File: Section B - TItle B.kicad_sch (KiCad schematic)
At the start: 2 parts

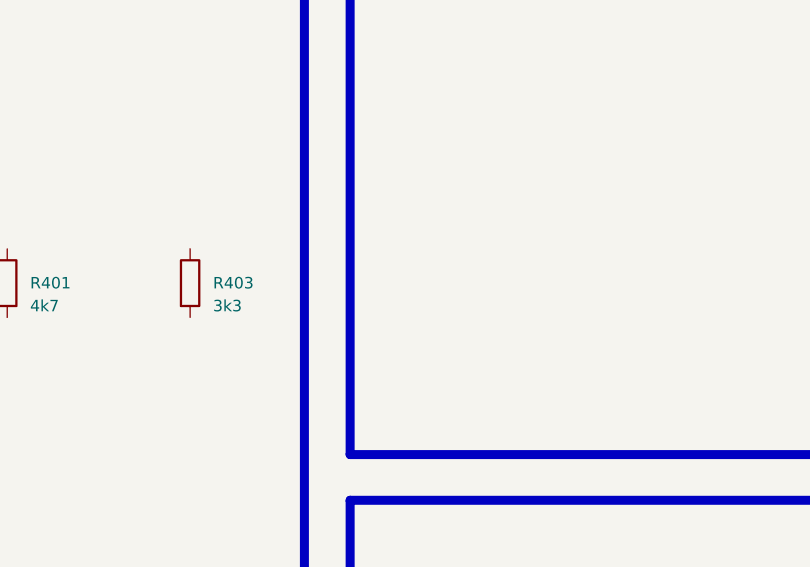
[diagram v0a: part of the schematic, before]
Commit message: section-a: grant myself all sheets, edit B
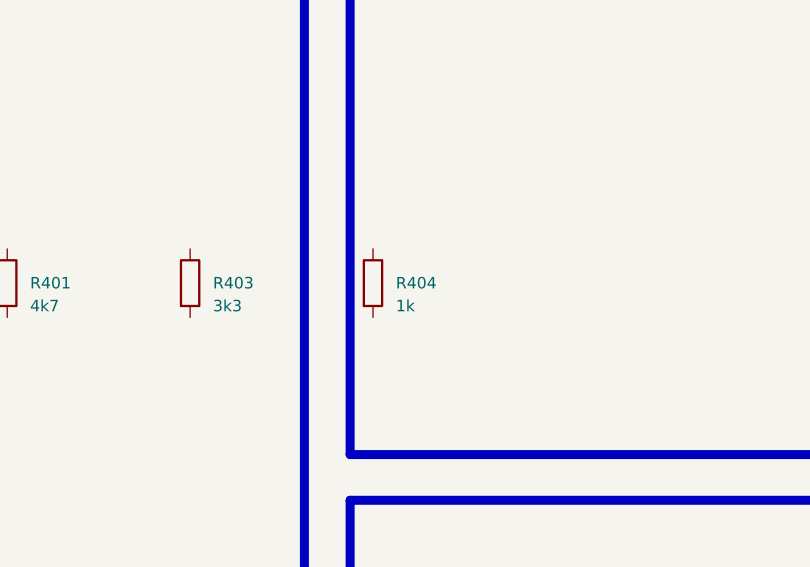
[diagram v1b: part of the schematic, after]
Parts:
- added R404: 1k, Resistor_SMD:R_0603_1608Metric, symbol Device:R
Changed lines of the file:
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@@
+		)
+	)
+	(symbol
+		(lib_id "Device:R")
+		(at 142.24 101.6 0)
+		(unit 1)
+		(exclude_from_sim no)
+		(in_bom yes)
+		(on_board yes)
+		(dnp no)
+		(property "Reference" "R404"
+			(at 144.78 101.6 0)
+			(effects (font (size 1.27 1.27)) (justify left))
+		)
+		(property "Value" "1k"
+			(at 144.78 104.14 0)
+			(effects (font (size 1.27 1.27)) (justify left))
+		)
+		(property "Footprint" "Resistor_SMD:R_0603_1608Metric"
+			(at 142.24 101.6 0)
+			(effects (font (size 1.27 1.27)) (hide yes))
+		)
+		(property "Datasheet" "~"
+			(at 142.24 101.6 0)
+			(effects (font (size 1.27 1.27)) (hide yes))
+		)
+		(pin "1")
+		(pin "2")
+		(instances
+			(project "ci_dummy"
+				(path "/f9e05184-c88b-4a88-ae9c-ab2bdb32be7c/c5103ceb-5325-4a84-a025-9638a412984e/e744f3ce-03a6-44a6-8792-1447ef232b9a"
+					(reference "R404")
+					(unit 1)
+				)
+			)
 		)
 	)
